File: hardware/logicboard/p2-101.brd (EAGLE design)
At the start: 72 x 72 mm, 41 parts, among them IC2 4066N, J1 MKR, J2 GPIO, J3 Vcc, J4 RLY, J5 SPI, J6 LED, K1 G5V1, T1 2SC1815, U1 DS18B20

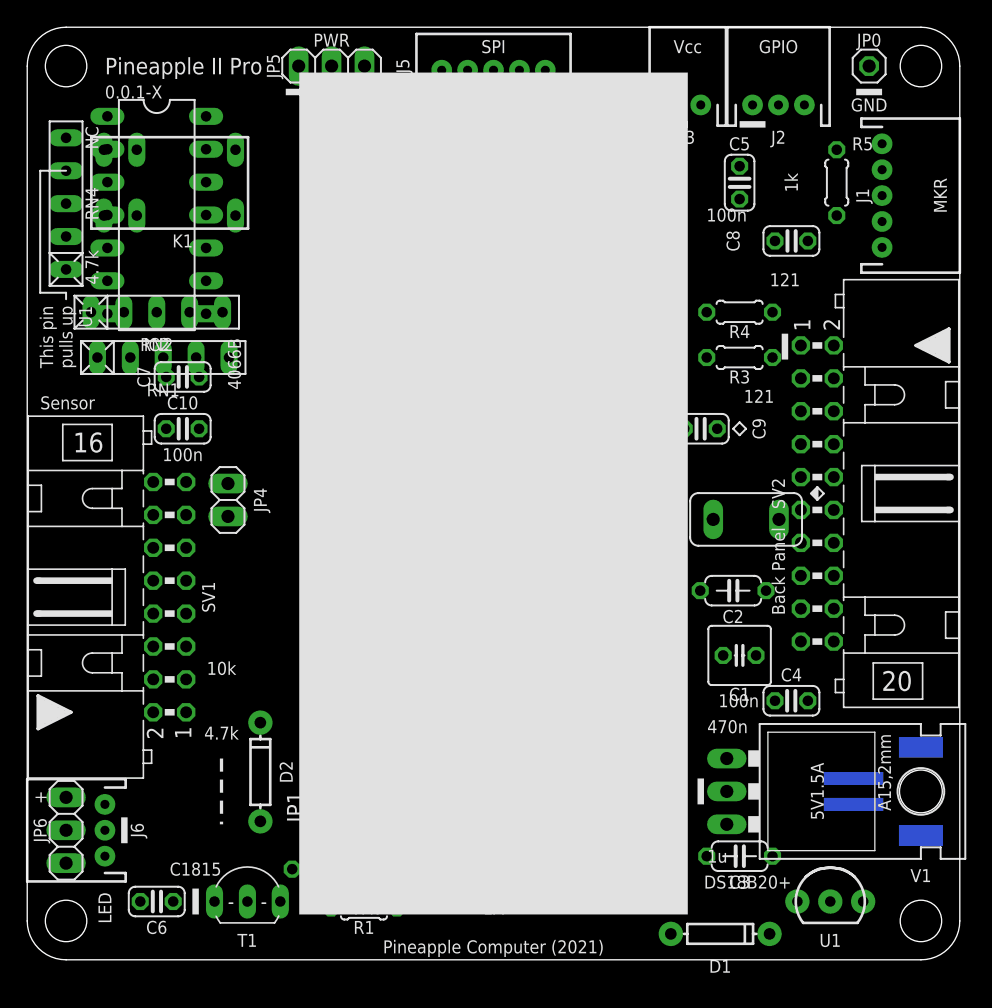
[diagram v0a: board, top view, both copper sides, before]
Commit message: Unknown...
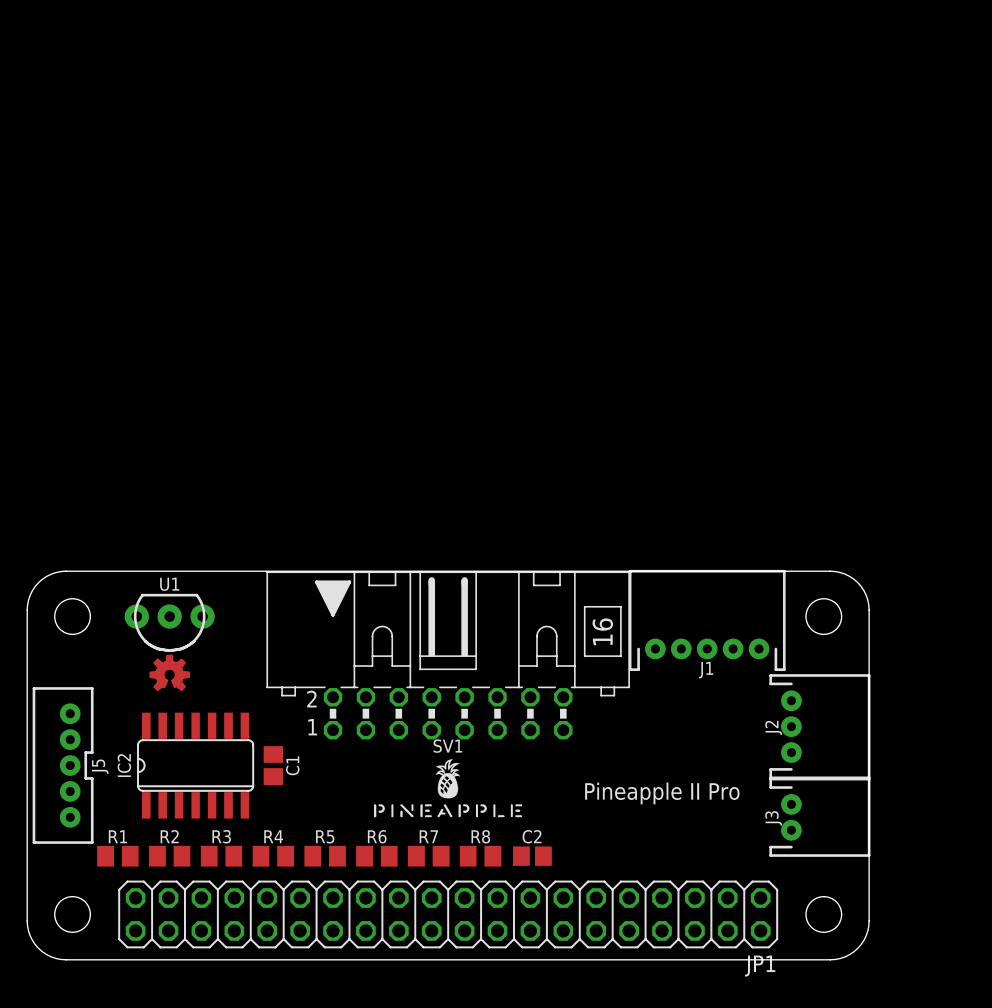
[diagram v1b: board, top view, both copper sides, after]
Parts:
- removed C10, C4, C5: 100n, rcl:C025-024X044
- removed C3: 1u, rcl:C050-024X044
- removed C6, C7, C8, C9: 10n, resistor:C025-024X044
- removed D1, D2: (no value), SparkFun-DiscreteSemi:DIODE-1N4148
- removed F1: 1.8A, fuse:TE5
- removed J4: RLY, SparkFun-Connectors:JST-2-SMD
- removed J6: LED, SparkFun-Connectors:JST-3-PTH
- removed JP0: GNDPIN, pinhead:1X01
- removed JP4: RLYJMP, pinhead:1X02
- removed JP5: D5V, pinhead:1X03
- removed JP6: LED, pinhead:1X03
- removed K1: G5V1, relay:G5V1
- removed RN1, RN4: 4.7k, resistor-net:RN-5
- removed RN2: 10k, resistor-net:RN-5
- removed SV2: (no value), con-ml:ML20L
- removed T1: 2SC1815, transistor:TO92-ECB
- removed V1: 5V, v-reg:78XXL
- added R6, R7, R8: (no value), rcl:M2012
- C1: value 22u -> (none); device rcl:C025-050X050 -> rcl:C2012
- C2: value 470n -> (none); device rcl:C050-024X044 -> rcl:C2012
- IC2: value 4066N -> 4066D; device 40xx:DIL14 -> 40xx:SO14
- R1: value 47k -> (none); device resistor:0204/5 -> rcl:M2012
- R2, R5: value 1k -> (none); device resistor:0204/5 -> rcl:M2012
- R3, R4: value 120 -> (none); device resistor:0204/5 -> rcl:M2012
- moved R5 65.3 mm to (23.0, 8.00), turned to 0 degrees
- moved J5 62.6 mm to (3.50, 15.0), turned to 90 degrees
- moved J3 55.6 mm to (59.0, 11.0), turned to 270 degrees
- moved U1 55.5 mm to (11.0, 26.5), turned to 180 degrees
- moved R3 55.5 mm to (15.0, 8.00)
- moved R4 55.3 mm to (19.0, 8.00)
- moved J2 48.0 mm to (59.0, 18.0), turned to 270 degrees
- moved IC2 42.6 mm to (13.0, 15.0), turned to 0 degrees
- moved J1 37.5 mm to (52.5, 24.0), turned to 0 degrees
- moved C1 37.0 mm to (19.0, 15.0), turned to 90 degrees
- moved JP1 33.5 mm to (32.5, 3.50), turned to 180 degrees
- moved LOGO1 28.7 mm to (11.0, 22.0)
- moved C2 25.7 mm to (39.0, 8.00)
- moved SV1 23.3 mm to (32.5, 19.0), turned to 0 degrees
- moved U$1 22.8 mm to (32.5, 11.0), flipped to the top
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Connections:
- removed net LED0: R4.2
- removed net LED0A: J6.1, JP6.1, R4.1, SV2.5
- removed net LED1: R3.2
- removed net LED1A: J6.3, JP6.3, R3.1
- removed net MIRTN: SV2.8
- removed net MISND: SV2.7
- removed net MORTN: SV2.14
- removed net MOSND: SV2.13
- removed net MRX+: SV2.9
- removed net MRX-: SV2.11
- removed net MRXDTCT: SV2.10
- removed net MTRTN: SV2.18
- removed net MTSND: SV2.17
- removed net MTX+: SV2.15
- removed net MTX-: SV2.16
- removed net NMO2RTN: RN1.5
- removed net NMORTN: RN1.4
- removed net NMTRTN: RN1.3
- removed net RLY: R2.2
- removed net RLYDRV: R1.2, R2.1, T1.B
- removed net RLYOUT: J4.2, K1.10
- removed net RLYSNK: D2.A, K1.9, T1.C
- removed net RST: SV2.3
- removed net V+: C1.1, C2.1, D1.C, JP5.3, SV2.2, V1.IN
- removed net VOUT: F1.2
- removed net VOUTRAW: C3.1, C4.1, D1.A, J4.1, JP4.2, K1.5, K1.6, V1.OUT
- removed net VOUTRAW2: F1.1, JP4.1, K1.1
- new net CE0: JP1.24
- new net CE1: JP1.26
- new net EEPROMSCL: JP1.28
- new net EEPROMSDA: JP1.27
- new net GPCLK0: JP1.7
- new net GPIO16: JP1.36
- new net GPIO17: JP1.11
- new net GPIO22: JP1.15
- new net GPIO23: JP1.16
- new net GPIO24: JP1.18
- new net GPIO25: JP1.22
- new net GPIO26: JP1.37
- new net GPIO27: JP1.13
- new net GPIO5: JP1.29
- new net GPIO6: JP1.31
- new net MISO0: JP1.21
- new net MOSI0: JP1.19
- new net PCMCLK: JP1.12
- new net PCMDIN: JP1.38
- new net PCMDOUT: JP1.40
- new net PCMFS: JP1.35
- new net PWM0: JP1.32
- new net PWM1: JP1.33
- new net SCL1: JP1.5
- new net SCLK0: JP1.23
- new net SDA1: JP1.3
- new net TX: JP1.8
- new net VDD: JP1.1, JP1.17
- net ANLG1: now also R1.2; no longer RN2.2
- net ANLG2: now also R2.2; no longer RN2.3
- net ANLG3: now also R3.2; no longer RN2.4
- net ANLG4: now also R4.2; no longer RN2.5
- net AREF: now also C2.1, R8.2; no longer C5.1, R5.1
- net GND: now also JP1.14, JP1.20, JP1.25, JP1.30, JP1.34, JP1.39, JP1.6, JP1.9, R2.1, R3.1, R4.1; no longer C10.2, C3.2, C4.2, C5.2, C6.2, C7.2, C8.2, C9.2, J6.2, JP0.1, JP5.1, JP6.2, RN2.1, SV2.1, SV2.12, SV2.20, SV2.4, SV2.6, T1.E, V1.GND
- net RX: now also JP1.10; no longer RN1.2
- net SCL: now also R6.2; no longer RN4.3
- net SDA: now also R5.2; no longer RN4.2
- net THS: now also R7.2; no longer RN4.4
- net VCC: now also C1.1, JP1.2, JP1.4, R5.1, R6.1, R7.1, R8.1; no longer C10.1, C6.1, C7.1, C8.1, C9.1, D2.C, JP5.2, K1.2, RN1.1, RN4.1, SV2.19
- net VCC/2: no longer R5.2
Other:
- board size 72 x 72 mm -> 65 x 30 mm
- board text removed: "*Cut pull-up R to install LM35"
- board text removed: "*Cut this pin to use LM35"
- board text removed: "+"
- board text removed: "0.0.1-X"
- board text removed: "100n"
- board text removed: "10k"
- board text removed: "121"
- board text removed: "1A"
- board text removed: "1k"
- board text removed: "1u"
- board text removed: "3V3"
- board text removed: "4.7k"
- board text removed: "4066B"
- board text removed: "470n"
- board text removed: "47k"
- board text removed: "5V1.5A"
- board text removed: "74153"
- board text removed: "Arduino"
- board text removed: "Back Panel"
- board text removed: "Bottom View"
- board text removed: "C"
- board text removed: "C1815"
- board text removed: "Close"
- board text removed: "D7"
- board text removed: "DS18B20+"
- board text removed: "Direct 5V"
- board text removed: "Don't Close"
- board text removed: "Dual"
- board text removed: "Ext. V+"
- board text removed: "G"
- board text removed: "G1"
- board text removed: "G2"
- board text removed: "GND"
- board text removed: "GPIO"
- board text removed: "I"
- board text removed: "IN-RX"
- board text removed: "Insulating Tape Here"
- board text removed: "LED"
- board text removed: "LED0"
- board text removed: "LED1"
- board text removed: "LTC485"
- board text removed: "MKR"
- board text removed: "NC"
- board text removed: "O"
- board text removed: "OUT2"
- board text removed: "Open JP1"
- board text removed: "PWR"
- board text removed: "PWRSEL"
- board text removed: "Pineapple Computer (2021)"
- board text removed: "Qwiic/5V"
- board text removed: "RLYJMP"
- board text removed: "RTN"
- board text removed: "RX"
- board text removed: "Regulator"
- board text removed: "Relay"
- board text removed: "SC"
- board text removed: "SCL"
- board text removed: "SD"
- board text removed: "SDA"
- board text removed: "SND"
- board text removed: "SPI"
- board text removed: "Sensor"
- board text removed: "TX"
- board text removed: "This pin pulls up U1"
- board text removed: "U1"
- board text removed: "V"
- board text removed: "V+"
- board text removed: "Vcc"
- board text removed: "Vcc/2"
- board text removed: "Vin"
- board text removed: "Vin (MC)"
- board text removed: "Vout"
- board text removed: "Vout (Reg)"
- board text removed: "Voutraw"
- board text removed: "You can istall LM35* instead of DS18B20+"
